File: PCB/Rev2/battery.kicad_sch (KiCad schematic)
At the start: 11 parts, among them U2 TP4057, U3 TPS2116DRL, U4 TPS2116DRL

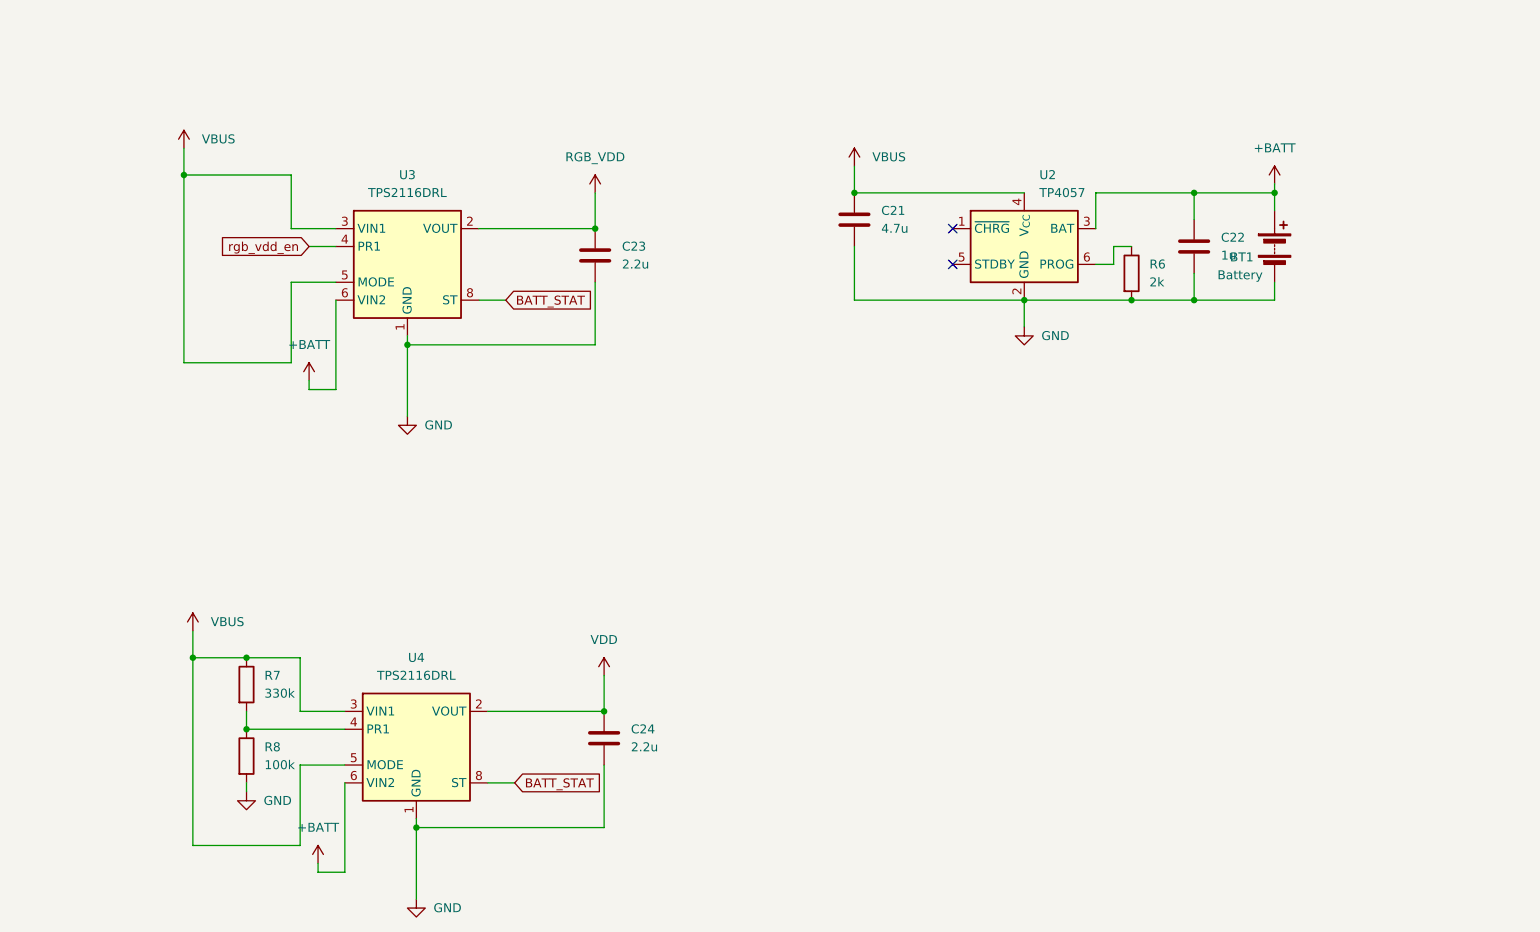
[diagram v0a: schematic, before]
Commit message: sc2最终审核（nayat）
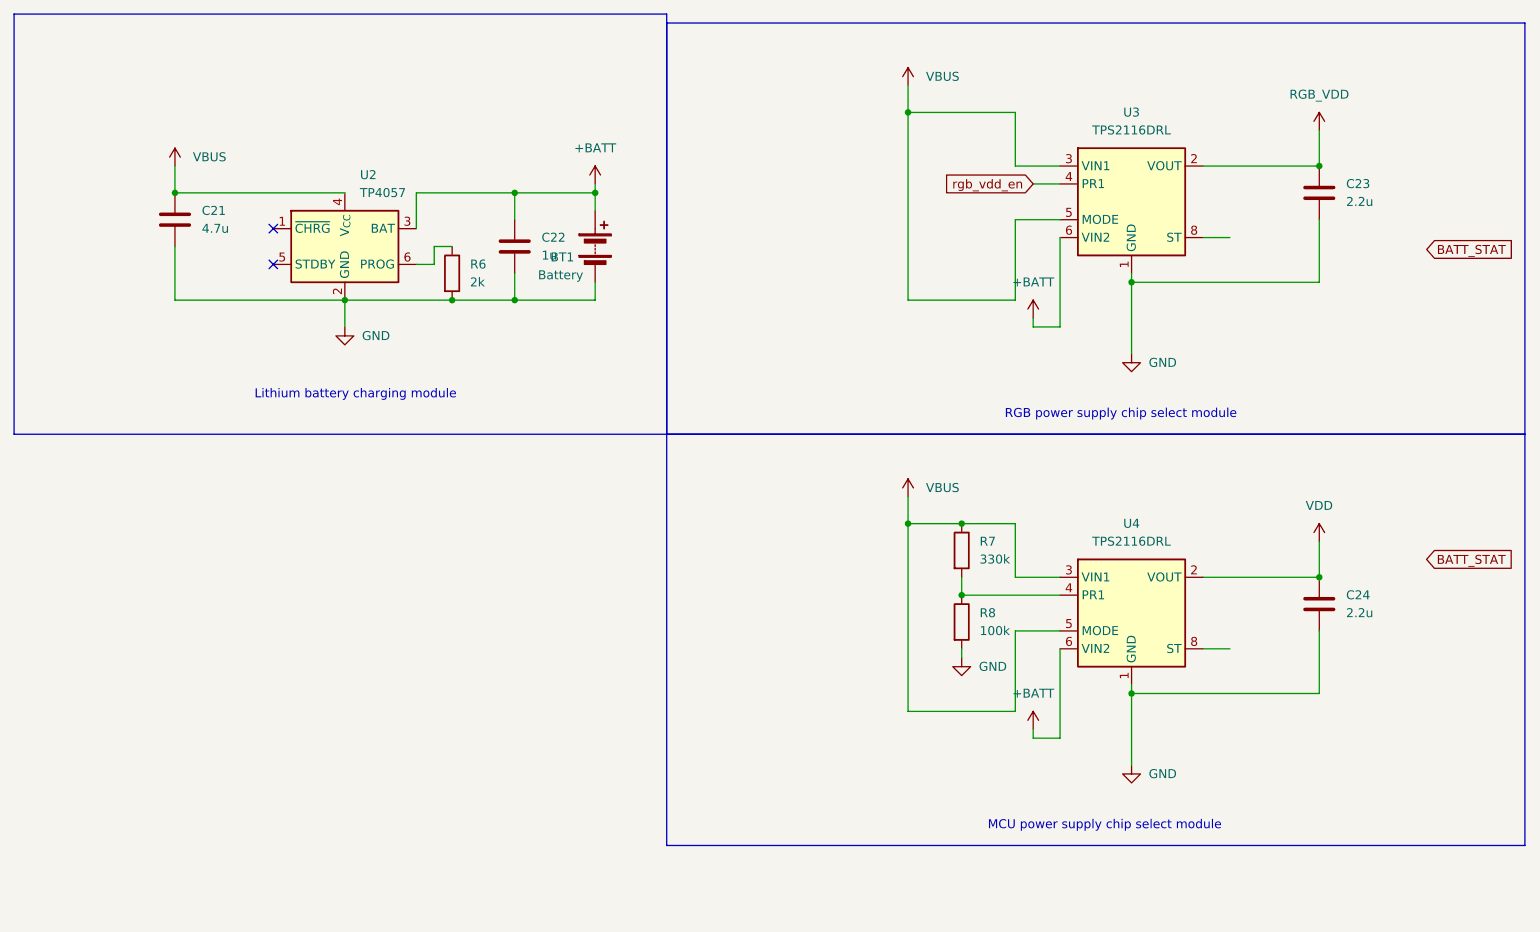
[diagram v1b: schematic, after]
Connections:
- net BATT_STAT: no longer U3.8 (ST), U4.8 (ST)
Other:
- note added: "Lithium battery charging module"
- note added: "MCU power supply chip select module"
- note added: "RGB power supply chip select module"
- moved on the sheet: BT1, C21, C22, C23, C24, R6, R7, R8, U2, U3, U4
